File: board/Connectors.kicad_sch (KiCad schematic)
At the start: 17 parts, among them J10 SLOT 1, J11 SLOT 2, J12 SLOT 3, J13 SLOT 4, J14 SLOT 5, J15 AudioJack3, J16 SPI Device 0, J18 SPI Device 1, J19 SPI Device 2, J20 SPI Device 3, J21 SPI Device 4, J22 SPI Device 5, J23 SPI Device 6, J24 SPI Device 7, J25 VIA Port A, J26 SP720APP, J9 SLOT 0

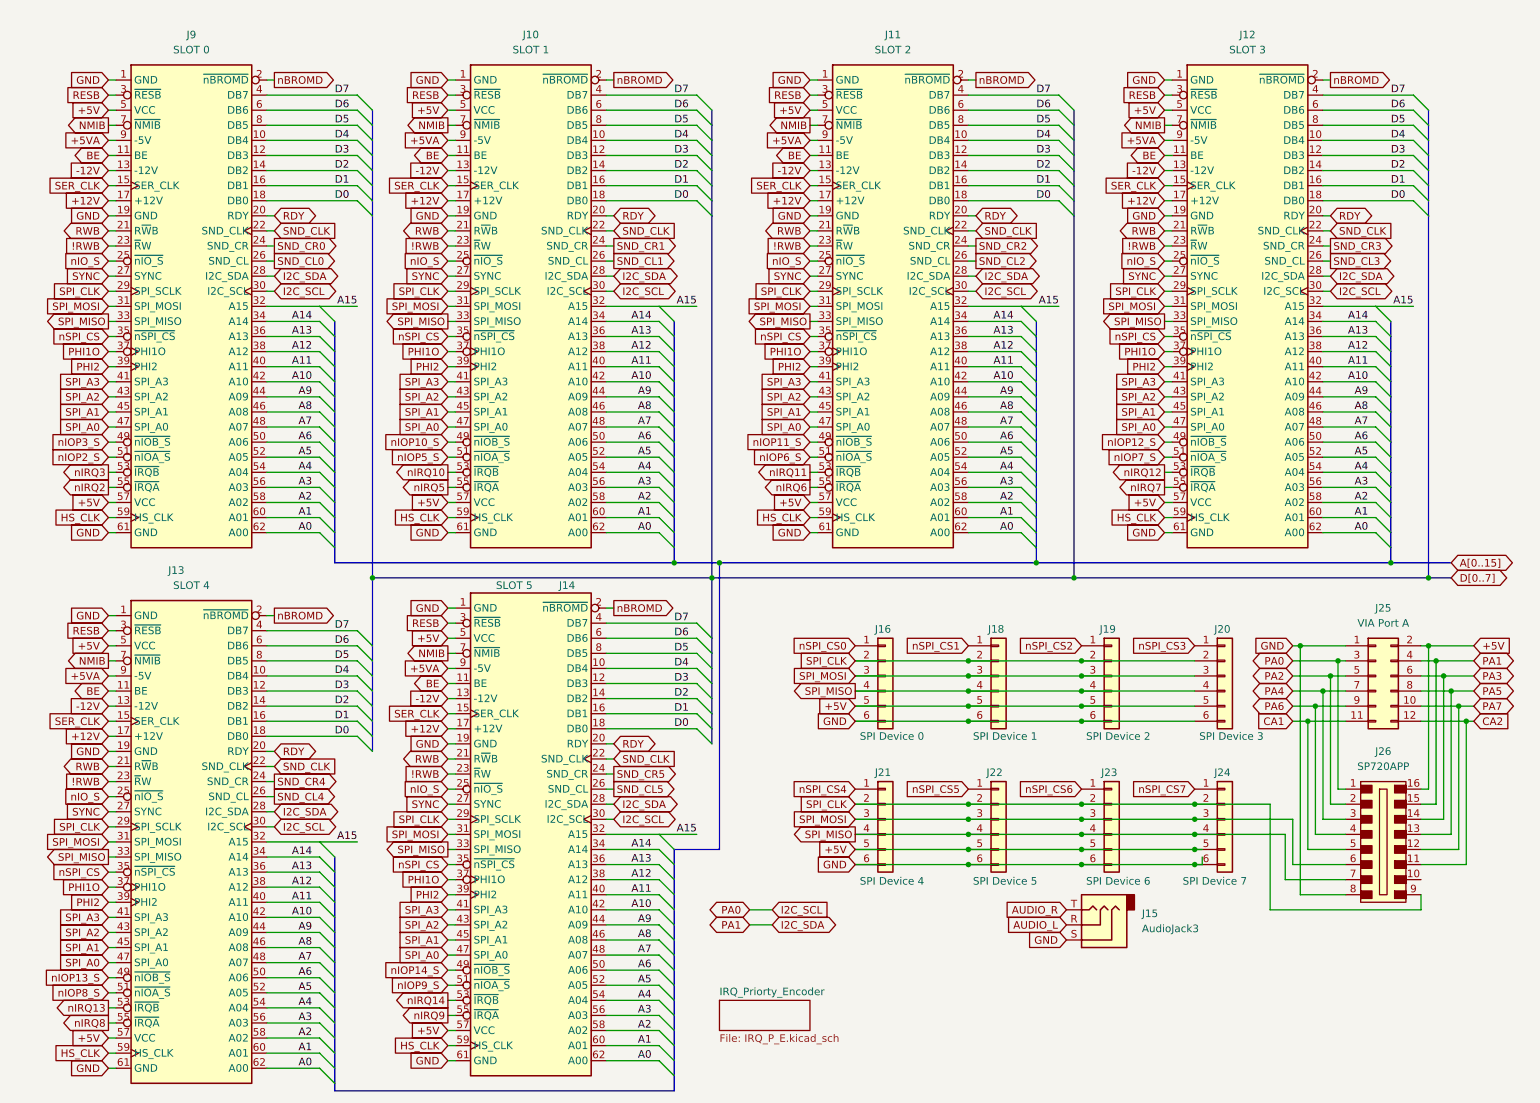
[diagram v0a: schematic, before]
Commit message: Board V1.1G
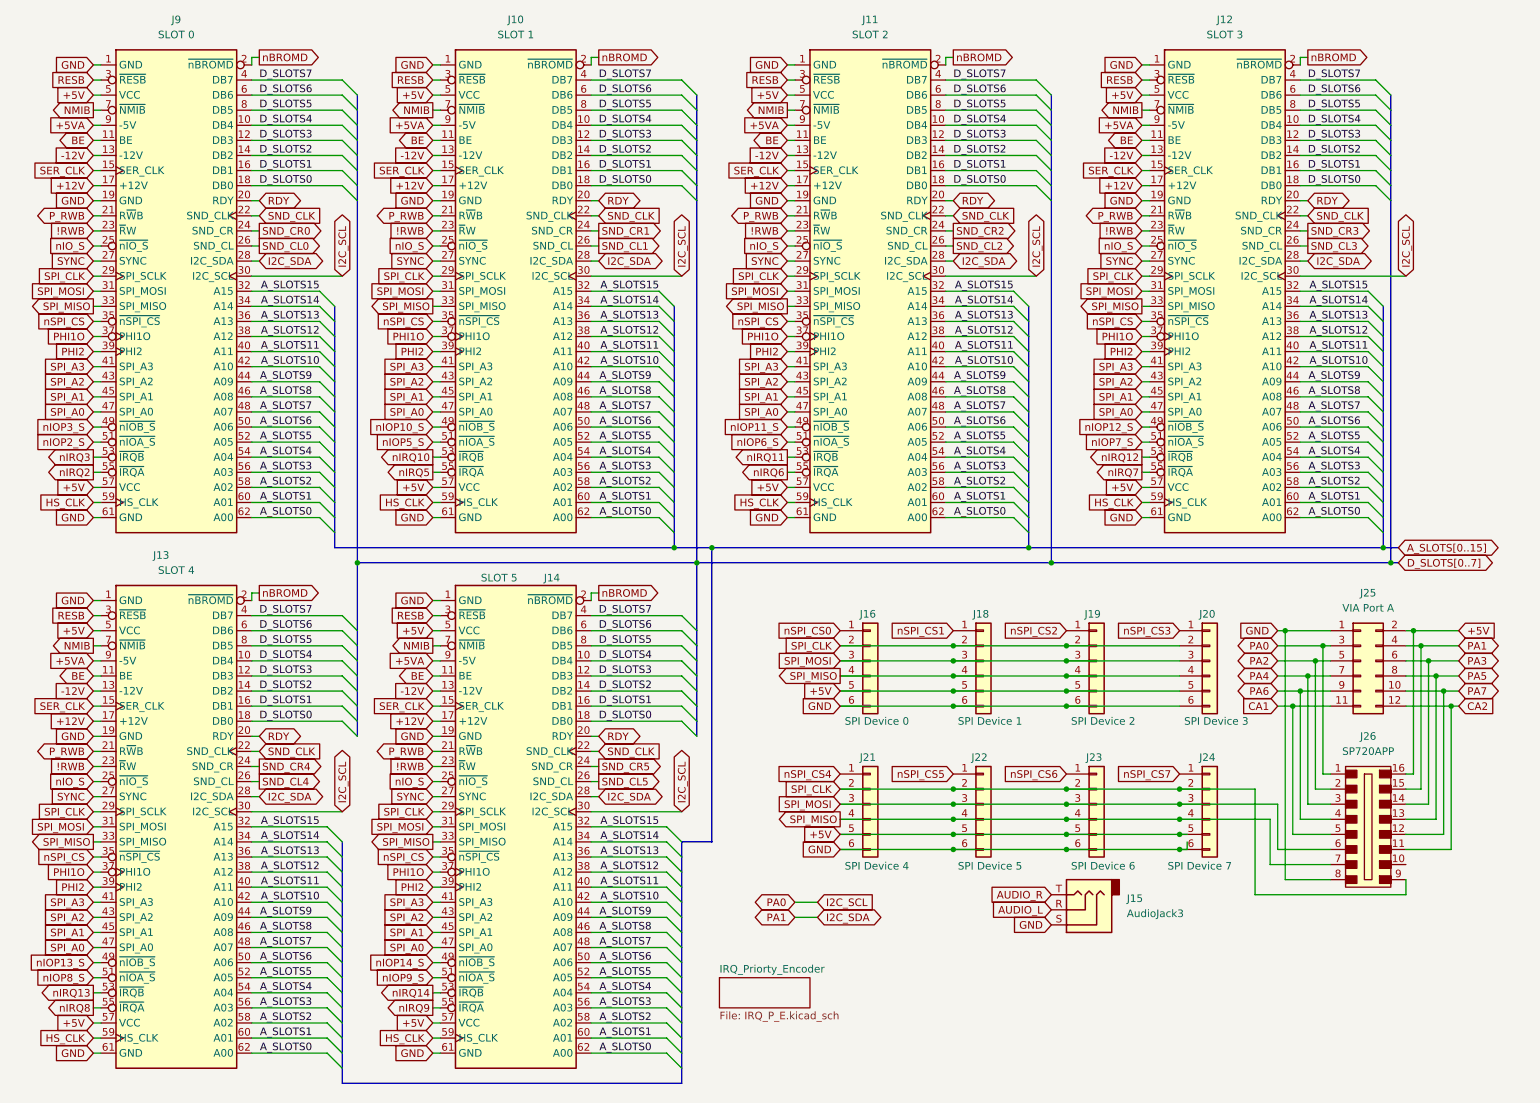
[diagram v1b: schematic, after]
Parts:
- J15: footprint Connector_Audio:Jack_3.5mm_CUI_SJ1-3523N_Horizontal -> Connector_Audio:Jack_3.5mm_CUI_SJ1-3525N_Horizontal
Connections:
- net A0 renamed A_SLOTS0
- net A1 renamed A_SLOTS1
- net A10 renamed A_SLOTS10
- net A11 renamed A_SLOTS11
- net A12 renamed A_SLOTS12
- net A13 renamed A_SLOTS13
- net A14 renamed A_SLOTS14
- net A15 renamed A_SLOTS15
- net A2 renamed A_SLOTS2
- net A3 renamed A_SLOTS3
- net A4 renamed A_SLOTS4
- net A5 renamed A_SLOTS5
- net A6 renamed A_SLOTS6
- net A7 renamed A_SLOTS7
- net A8 renamed A_SLOTS8
- net A9 renamed A_SLOTS9
- net D0 renamed D_SLOTS0
- net D1 renamed D_SLOTS1
- net D2 renamed D_SLOTS2
- net D3 renamed D_SLOTS3
- net D4 renamed D_SLOTS4
- net D5 renamed D_SLOTS5
- net D6 renamed D_SLOTS6
- net D7 renamed D_SLOTS7
- net RWB renamed P_RWB
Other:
- moved on the sheet: J10, J11, J12, J13, J14, J15, J16, J18, J19, J20, J21, J22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
